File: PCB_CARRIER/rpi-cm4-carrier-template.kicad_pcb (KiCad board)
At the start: 2 copper layers, 40 x 55 mm, 1 part

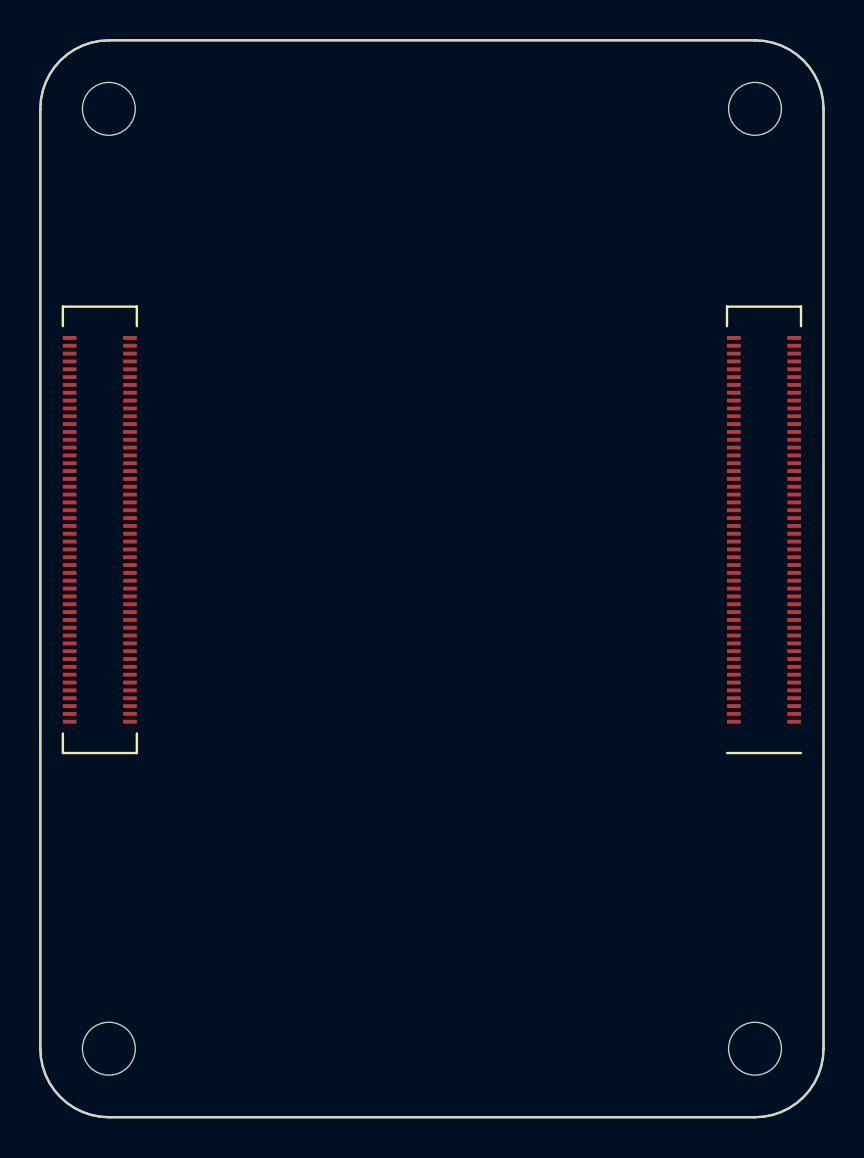
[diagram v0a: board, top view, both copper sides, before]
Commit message: upgrading the template files to newest kicad
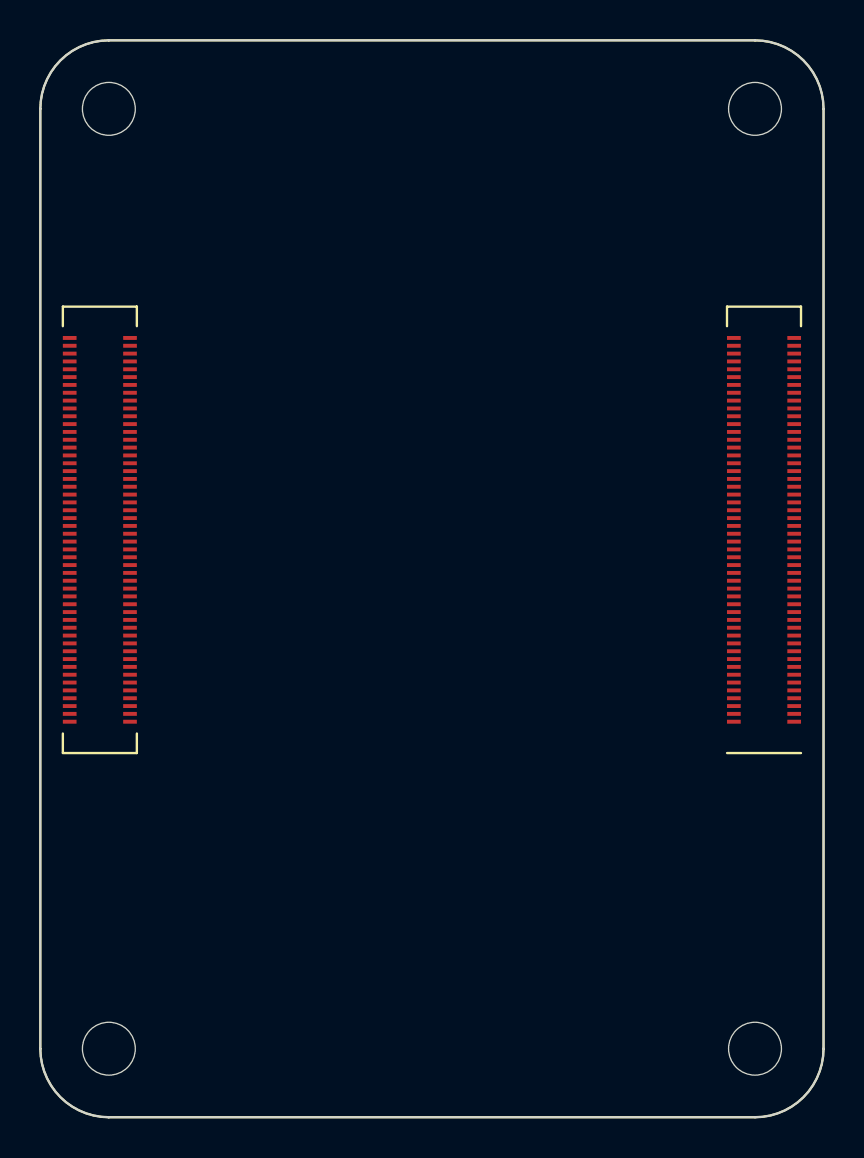
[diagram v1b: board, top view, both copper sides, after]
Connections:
- Module1 pad 1: Net-(Module1-Pad1) -> GND
- Module1 pad 10: Net-(Module1-Pad10) -> unconnected-(Module1A-Ethernet_Pair0_N-Pad10)
- Module1 pad 100: Net-(Module1-Pad100) -> unconnected-(Module1A-nEXTRST-Pad100)
- Module1 pad 101: Net-(Module1-Pad101) -> unconnected-(Module1B-USB_OTG_ID-Pad101)
- Module1 pad 102: Net-(Module1-Pad102) -> unconnected-(Module1B-PCIe_CLK_nREQ-Pad102)
- Module1 pad 103: Net-(Module1-Pad103) -> unconnected-(Module1B-USB2_N-Pad103)
- Module1 pad 104: Net-(Module1-Pad104) -> unconnected-(Module1B-Reserved-Pad104)
- Module1 pad 105: Net-(Module1-Pad105) -> unconnected-(Module1B-USB2_P-Pad105)
- Module1 pad 106: Net-(Module1-Pad106) -> unconnected-(Module1B-Reserved-Pad106)
- Module1 pad 107: Net-(Module1-Pad107) -> GND
- Module1 pad 108: Net-(Module1-Pad108) -> GND
- Module1 pad 109: Net-(Module1-Pad109) -> unconnected-(Module1B-PCIe_nRST-Pad109)
- Module1 pad 11: Net-(Module1-Pad11) -> unconnected-(Module1A-Ethernet_Pair2_P-Pad11)
- Module1 pad 110: Net-(Module1-Pad110) -> unconnected-(Module1B-PCIe_CLK_P-Pad110)
- Module1 pad 111: Net-(Module1-Pad111) -> unconnected-(Module1B-VDAC_COMP-Pad111)
- Module1 pad 112: Net-(Module1-Pad112) -> unconnected-(Module1B-PCIe_CLK_N-Pad112)
- Module1 pad 113: Net-(Module1-Pad113) -> GND
- Module1 pad 114: Net-(Module1-Pad114) -> GND
- Module1 pad 115: Net-(Module1-Pad115) -> unconnected-(Module1B-CAM1_D0_N-Pad115)
- Module1 pad 116: Net-(Module1-Pad116) -> unconnected-(Module1B-PCIe_RX_P-Pad116)
- Module1 pad 117: Net-(Module1-Pad117) -> unconnected-(Module1B-CAM1_D0_P-Pad117)
- Module1 pad 118: Net-(Module1-Pad118) -> unconnected-(Module1B-PCIe_RX_N-Pad118)
- Module1 pad 119: Net-(Module1-Pad119) -> GND
- Module1 pad 12: Net-(Module1-Pad12) -> unconnected-(Module1A-Ethernet_Pair0_P-Pad12)
- Module1 pad 120: Net-(Module1-Pad120) -> GND
- Module1 pad 121: Net-(Module1-Pad121) -> unconnected-(Module1B-CAM1_D1_N-Pad121)
- Module1 pad 122: Net-(Module1-Pad122) -> unconnected-(Module1B-PCIe_TX_P-Pad122)
- Module1 pad 123: Net-(Module1-Pad123) -> unconnected-(Module1B-CAM1_D1_P-Pad123)
- Module1 pad 124: Net-(Module1-Pad124) -> unconnected-(Module1B-PCIe_TX_N-Pad124)
- Module1 pad 125: Net-(Module1-Pad125) -> GND
- Module1 pad 126: Net-(Module1-Pad126) -> GND
- Module1 pad 127: Net-(Module1-Pad127) -> unconnected-(Module1B-CAM1_C_N-Pad127)
- Module1 pad 128: Net-(Module1-Pad128) -> unconnected-(Module1B-CAM0_D0_N-Pad128)
- Module1 pad 129: Net-(Module1-Pad129) -> unconnected-(Module1B-CAM1_C_P-Pad129)
- Module1 pad 13: Net-(Module1-Pad13) -> GND
- Module1 pad 130: Net-(Module1-Pad130) -> unconnected-(Module1B-CAM0_D0_P-Pad130)
- Module1 pad 131: Net-(Module1-Pad131) -> GND
- Module1 pad 132: Net-(Module1-Pad132) -> GND
- Module1 pad 133: Net-(Module1-Pad133) -> unconnected-(Module1B-CAM1_D2_N-Pad133)
- Module1 pad 134: Net-(Module1-Pad134) -> unconnected-(Module1B-CAM0_D1_N-Pad134)
- Module1 pad 135: Net-(Module1-Pad135) -> unconnected-(Module1B-CAM1_D2_P-Pad135)
- Module1 pad 136: Net-(Module1-Pad136) -> unconnected-(Module1B-CAM0_D1_P-Pad136)
- Module1 pad 137: Net-(Module1-Pad137) -> GND
- Module1 pad 138: Net-(Module1-Pad138) -> GND
- Module1 pad 139: Net-(Module1-Pad139) -> unconnected-(Module1B-CAM1_D3_N-Pad139)
- Module1 pad 14: Net-(Module1-Pad14) -> GND
- Module1 pad 140: Net-(Module1-Pad140) -> unconnected-(Module1B-CAM0_C_N-Pad140)
- Module1 pad 141: Net-(Module1-Pad141) -> unconnected-(Module1B-CAM1_D3_P-Pad141)
- Module1 pad 142: Net-(Module1-Pad142) -> unconnected-(Module1B-CAM0_C_P-Pad142)
- Module1 pad 143: Net-(Module1-Pad143) -> unconnected-(Module1B-HDMI1_HOTPLUG-Pad143)
- Module1 pad 144: Net-(Module1-Pad144) -> GND
- Module1 pad 145: Net-(Module1-Pad145) -> unconnected-(Module1B-HDMI1_SDA-Pad145)
- Module1 pad 146: Net-(Module1-Pad146) -> unconnected-(Module1B-HDMI1_TX2_P-Pad146)
- Module1 pad 147: Net-(Module1-Pad147) -> unconnected-(Module1B-HDMI1_SCL-Pad147)
- Module1 pad 148: Net-(Module1-Pad148) -> unconnected-(Module1B-HDMI1_TX2_N-Pad148)
- Module1 pad 149: Net-(Module1-Pad149) -> unconnected-(Module1B-HDMI1_CEC-Pad149)
- Module1 pad 15: Net-(Module1-Pad15) -> unconnected-(Module1A-Ethernet_nLED3(3.3v)-Pad15)
- Module1 pad 150: Net-(Module1-Pad150) -> GND
- Module1 pad 151: Net-(Module1-Pad151) -> unconnected-(Module1B-HDMI0_CEC-Pad151)
- Module1 pad 152: Net-(Module1-Pad152) -> unconnected-(Module1B-HDMI1_TX1_P-Pad152)
- Module1 pad 153: Net-(Module1-Pad153) -> unconnected-(Module1B-HDMI0_HOTPLUG-Pad153)
- Module1 pad 154: Net-(Module1-Pad154) -> unconnected-(Module1B-HDMI1_TX1_N-Pad154)
- Module1 pad 155: Net-(Module1-Pad155) -> GND
- Module1 pad 156: Net-(Module1-Pad156) -> GND
- Module1 pad 157: Net-(Module1-Pad157) -> unconnected-(Module1B-DSI0_D0_N-Pad157)
- Module1 pad 158: Net-(Module1-Pad158) -> unconnected-(Module1B-HDMI1_TX0_P-Pad158)
- Module1 pad 159: Net-(Module1-Pad159) -> unconnected-(Module1B-DSI0_D0_P-Pad159)
- Module1 pad 16: Net-(Module1-Pad16) -> unconnected-(Module1A-Ethernet_SYNC_IN(1.8v)-Pad16)
- Module1 pad 160: Net-(Module1-Pad160) -> unconnected-(Module1B-HDMI1_TX0_N-Pad160)
- Module1 pad 161: Net-(Module1-Pad161) -> GND
- Module1 pad 162: Net-(Module1-Pad162) -> GND
- Module1 pad 163: Net-(Module1-Pad163) -> unconnected-(Module1B-DSI0_D1_N-Pad163)
- Module1 pad 164: Net-(Module1-Pad164) -> unconnected-(Module1B-HDMI1_CLK_P-Pad164)
- Module1 pad 165: Net-(Module1-Pad165) -> unconnected-(Module1B-DSI0_D1_P-Pad165)
- Module1 pad 166: Net-(Module1-Pad166) -> unconnected-(Module1B-HDMI1_CLK_N-Pad166)
- Module1 pad 167: Net-(Module1-Pad167) -> GND
- Module1 pad 168: Net-(Module1-Pad168) -> GND
- Module1 pad 169: Net-(Module1-Pad169) -> unconnected-(Module1B-DSI0_C_N-Pad169)
- Module1 pad 17: Net-(Module1-Pad17) -> unconnected-(Module1A-Ethernet_nLED2(3.3v)-Pad17)
- Module1 pad 170: Net-(Module1-Pad170) -> unconnected-(Module1B-HDMI0_TX2_P-Pad170)
- Module1 pad 171: Net-(Module1-Pad171) -> unconnected-(Module1B-DSI0_C_P-Pad171)
- Module1 pad 172: Net-(Module1-Pad172) -> unconnected-(Module1B-HDMI0_TX2_N-Pad172)
- Module1 pad 173: Net-(Module1-Pad173) -> GND
- Module1 pad 174: Net-(Module1-Pad174) -> GND
- Module1 pad 175: Net-(Module1-Pad175) -> unconnected-(Module1B-DSI1_D0_N-Pad175)
- Module1 pad 176: Net-(Module1-Pad176) -> unconnected-(Module1B-HDMI0_TX1_P-Pad176)
- Module1 pad 177: Net-(Module1-Pad177) -> unconnected-(Module1B-DSI1_D0_P-Pad177)
- Module1 pad 178: Net-(Module1-Pad178) -> unconnected-(Module1B-HDMI0_TX1_N-Pad178)
- Module1 pad 179: Net-(Module1-Pad179) -> GND
- Module1 pad 18: Net-(Module1-Pad18) -> unconnected-(Module1A-Ethernet_SYNC_OUT(1.8v)-Pad18)
- Module1 pad 180: Net-(Module1-Pad180) -> GND
- Module1 pad 181: Net-(Module1-Pad181) -> unconnected-(Module1B-DSI1_D1_N-Pad181)
- Module1 pad 182: Net-(Module1-Pad182) -> unconnected-(Module1B-HDMI0_TX0_P-Pad182)
- Module1 pad 183: Net-(Module1-Pad183) -> unconnected-(Module1B-DSI1_D1_P-Pad183)
- Module1 pad 184: Net-(Module1-Pad184) -> unconnected-(Module1B-HDMI0_TX0_N-Pad184)
- Module1 pad 185: Net-(Module1-Pad185) -> GND
- Module1 pad 186: Net-(Module1-Pad186) -> GND
- Module1 pad 187: Net-(Module1-Pad187) -> unconnected-(Module1B-DSI1_C_N-Pad187)
- Module1 pad 188: Net-(Module1-Pad188) -> unconnected-(Module1B-HDMI0_CLK_P-Pad188)
- Module1 pad 189: Net-(Module1-Pad189) -> unconnected-(Module1B-DSI1_C_P-Pad189)
- Module1 pad 19: Net-(Module1-Pad19) -> unconnected-(Module1A-Ethernet_nLED1(3.3v)-Pad19)
- Module1 pad 190: Net-(Module1-Pad190) -> unconnected-(Module1B-HDMI0_CLK_N-Pad190)
- Module1 pad 191: Net-(Module1-Pad191) -> GND
- Module1 pad 192: Net-(Module1-Pad192) -> GND
- Module1 pad 193: Net-(Module1-Pad193) -> unconnected-(Module1B-DSI1_D2_N-Pad193)
- Module1 pad 194: Net-(Module1-Pad194) -> unconnected-(Module1B-DSI1_D3_N-Pad194)
- Module1 pad 195: Net-(Module1-Pad195) -> unconnected-(Module1B-DSI1_D2_P-Pad195)
- Module1 pad 196: Net-(Module1-Pad196) -> unconnected-(Module1B-DSI1_D3_P-Pad196)
- Module1 pad 197: Net-(Module1-Pad197) -> GND
- Module1 pad 198: Net-(Module1-Pad198) -> GND
- Module1 pad 199: Net-(Module1-Pad199) -> unconnected-(Module1B-HDMI0_SDA-Pad199)
- Module1 pad 2: Net-(Module1-Pad2) -> GND
- Module1 pad 20: Net-(Module1-Pad20) -> unconnected-(Module1A-EEPROM_nWP-Pad20)
- Module1 pad 200: Net-(Module1-Pad200) -> unconnected-(Module1B-HDMI0_SCL-Pad200)
- Module1 pad 21: Net-(Module1-Pad21) -> unconnected-(Module1A-PI_nLED_Activity-Pad21)
- Module1 pad 22: Net-(Module1-Pad22) -> GND
- Module1 pad 23: Net-(Module1-Pad23) -> GND
- Module1 pad 24: Net-(Module1-Pad24) -> unconnected-(Module1A-GPIO26-Pad24)
- Module1 pad 25: Net-(Module1-Pad25) -> unconnected-(Module1A-GPIO21-Pad25)
- Module1 pad 26: Net-(Module1-Pad26) -> unconnected-(Module1A-GPIO19-Pad26)
- Module1 pad 27: Net-(Module1-Pad27) -> unconnected-(Module1A-GPIO20-Pad27)
- Module1 pad 28: Net-(Module1-Pad28) -> unconnected-(Module1A-GPIO13-Pad28)
- Module1 pad 29: Net-(Module1-Pad29) -> unconnected-(Module1A-GPIO16-Pad29)
- Module1 pad 3: Net-(Module1-Pad3) -> unconnected-(Module1A-Ethernet_Pair3_P-Pad3)
- Module1 pad 30: Net-(Module1-Pad30) -> unconnected-(Module1A-GPIO6-Pad30)
- Module1 pad 31: Net-(Module1-Pad31) -> unconnected-(Module1A-GPIO12-Pad31)
- Module1 pad 32: Net-(Module1-Pad32) -> GND
- Module1 pad 33: Net-(Module1-Pad33) -> GND
- Module1 pad 34: Net-(Module1-Pad34) -> unconnected-(Module1A-GPIO5-Pad34)
- Module1 pad 35: Net-(Module1-Pad35) -> unconnected-(Module1A-ID_SC-Pad35)
- Module1 pad 36: Net-(Module1-Pad36) -> unconnected-(Module1A-ID_SD-Pad36)
- Module1 pad 37: Net-(Module1-Pad37) -> unconnected-(Module1A-GPIO7-Pad37)
- Module1 pad 38: Net-(Module1-Pad38) -> unconnected-(Module1A-GPIO11-Pad38)
- Module1 pad 39: Net-(Module1-Pad39) -> unconnected-(Module1A-GPIO8-Pad39)
- Module1 pad 4: Net-(Module1-Pad4) -> unconnected-(Module1A-Ethernet_Pair1_P-Pad4)
- Module1 pad 40: Net-(Module1-Pad40) -> unconnected-(Module1A-GPIO9-Pad40)
- Module1 pad 41: Net-(Module1-Pad41) -> unconnected-(Module1A-GPIO25-Pad41)
- Module1 pad 42: Net-(Module1-Pad42) -> GND
- Module1 pad 43: Net-(Module1-Pad43) -> GND
- Module1 pad 44: Net-(Module1-Pad44) -> unconnected-(Module1A-GPIO10-Pad44)
- Module1 pad 45: Net-(Module1-Pad45) -> unconnected-(Module1A-GPIO24-Pad45)
- Module1 pad 46: Net-(Module1-Pad46) -> unconnected-(Module1A-GPIO22-Pad46)
- Module1 pad 47: Net-(Module1-Pad47) -> unconnected-(Module1A-GPIO23-Pad47)
- Module1 pad 48: Net-(Module1-Pad48) -> unconnected-(Module1A-GPIO27-Pad48)
- Module1 pad 49: Net-(Module1-Pad49) -> unconnected-(Module1A-GPIO18-Pad49)
- Module1 pad 5: Net-(Module1-Pad5) -> unconnected-(Module1A-Ethernet_Pair3_N-Pad5)
- Module1 pad 50: Net-(Module1-Pad50) -> unconnected-(Module1A-GPIO17-Pad50)
- Module1 pad 51: Net-(Module1-Pad51) -> unconnected-(Module1A-GPIO15-Pad51)
- Module1 pad 52: Net-(Module1-Pad52) -> GND
- Module1 pad 53: Net-(Module1-Pad53) -> GND
- Module1 pad 54: Net-(Module1-Pad54) -> unconnected-(Module1A-GPIO4-Pad54)
- Module1 pad 55: Net-(Module1-Pad55) -> unconnected-(Module1A-GPIO14-Pad55)
- Module1 pad 56: Net-(Module1-Pad56) -> unconnected-(Module1A-GPIO3-Pad56)
- Module1 pad 57: Net-(Module1-Pad57) -> unconnected-(Module1A-SD_CLK-Pad57)
- Module1 pad 58: Net-(Module1-Pad58) -> unconnected-(Module1A-GPIO2-Pad58)
- Module1 pad 59: Net-(Module1-Pad59) -> GND
- Module1 pad 6: Net-(Module1-Pad6) -> unconnected-(Module1A-Ethernet_Pair1_N-Pad6)
- Module1 pad 60: Net-(Module1-Pad60) -> GND
- Module1 pad 61: Net-(Module1-Pad61) -> unconnected-(Module1A-SD_DAT3-Pad61)
- Module1 pad 62: Net-(Module1-Pad62) -> unconnected-(Module1A-SD_CMD-Pad62)
- Module1 pad 63: Net-(Module1-Pad63) -> unconnected-(Module1A-SD_DAT0-Pad63)
- Module1 pad 64: Net-(Module1-Pad64) -> unconnected-(Module1A-SD_DAT5-Pad64)
- Module1 pad 65: Net-(Module1-Pad65) -> GND
- Module1 pad 66: Net-(Module1-Pad66) -> GND
- Module1 pad 67: Net-(Module1-Pad67) -> unconnected-(Module1A-SD_DAT1-Pad67)
- Module1 pad 68: Net-(Module1-Pad68) -> unconnected-(Module1A-SD_DAT4-Pad68)
- Module1 pad 69: Net-(Module1-Pad69) -> unconnected-(Module1A-SD_DAT2-Pad69)
- Module1 pad 7: Net-(Module1-Pad7) -> GND
- Module1 pad 70: Net-(Module1-Pad70) -> unconnected-(Module1A-SD_DAT7-Pad70)
- Module1 pad 71: Net-(Module1-Pad71) -> GND
- Module1 pad 72: Net-(Module1-Pad72) -> unconnected-(Module1A-SD_DAT6-Pad72)
- Module1 pad 73: Net-(Module1-Pad73) -> unconnected-(Module1A-SD_VDD_Override-Pad73)
- Module1 pad 74: Net-(Module1-Pad74) -> GND
- Module1 pad 75: Net-(Module1-Pad75) -> unconnected-(Module1A-SD_PWR_ON-Pad75)
- Module1 pad 76: Net-(Module1-Pad76) -> unconnected-(Module1A-Reserved-Pad76)
- Module1 pad 77: Net-(Module1-Pad77) -> +5V
- Module1 pad 78: Net-(Module1-Pad78) -> unconnected-(Module1A-GPIO_VREF(1.8v/3.3v_Input)-Pad78)
- Module1 pad 79: Net-(Module1-Pad79) -> +5V
- Module1 pad 8: Net-(Module1-Pad8) -> GND
- Module1 pad 80: Net-(Module1-Pad80) -> unconnected-(Module1A-SCL0-Pad80)
- Module1 pad 81: Net-(Module1-Pad81) -> +5V
- Module1 pad 82: Net-(Module1-Pad82) -> unconnected-(Module1A-SDA0-Pad82)
- Module1 pad 83: Net-(Module1-Pad83) -> +5V
- Module1 pad 84: Net-(Module1-Pad84) -> +3.3V
- Module1 pad 85: Net-(Module1-Pad85) -> +5V
- Module1 pad 86: Net-(Module1-Pad86) -> +3.3V
- Module1 pad 87: Net-(Module1-Pad87) -> +5V
- Module1 pad 88: Net-(Module1-Pad88) -> +1.8V
- Module1 pad 89: Net-(Module1-Pad89) -> unconnected-(Module1A-WiFi_nDisable-Pad89)
- Module1 pad 9: Net-(Module1-Pad9) -> unconnected-(Module1A-Ethernet_Pair2_N-Pad9)
- Module1 pad 90: Net-(Module1-Pad90) -> +1.8V
- Module1 pad 91: Net-(Module1-Pad91) -> unconnected-(Module1A-BT_nDisable-Pad91)
- Module1 pad 92: Net-(Module1-Pad92) -> unconnected-(Module1A-RUN_PG-Pad92)
- Module1 pad 93: Net-(Module1-Pad93) -> unconnected-(Module1A-nRPIBOOT-Pad93)
- Module1 pad 94: Net-(Module1-Pad94) -> unconnected-(Module1A-AnalogIP0-Pad94)
- Module1 pad 95: Net-(Module1-Pad95) -> unconnected-(Module1A-nPI_LED_PWR-Pad95)
- Module1 pad 96: Net-(Module1-Pad96) -> unconnected-(Module1A-AnalogIP1-Pad96)
- Module1 pad 97: Net-(Module1-Pad97) -> unconnected-(Module1A-Camera_GPIO-Pad97)
- Module1 pad 98: Net-(Module1-Pad98) -> GND
- Module1 pad 99: Net-(Module1-Pad99) -> unconnected-(Module1A-Global_EN-Pad99)
